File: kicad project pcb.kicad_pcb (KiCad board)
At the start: 2 copper layers, 35.3 x 38.9 mm, 11 parts, among them J1 Jack-DC, J2 Screw_Terminal_01x02, Q1 2N7000

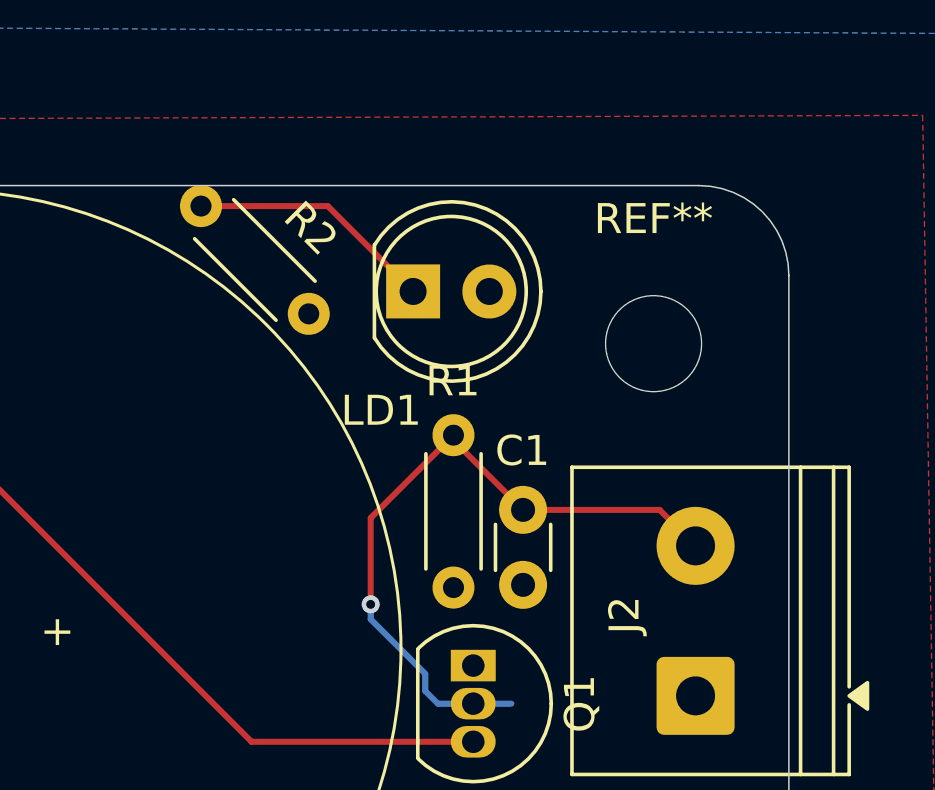
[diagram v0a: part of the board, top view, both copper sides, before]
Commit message: Update LED and screenshots
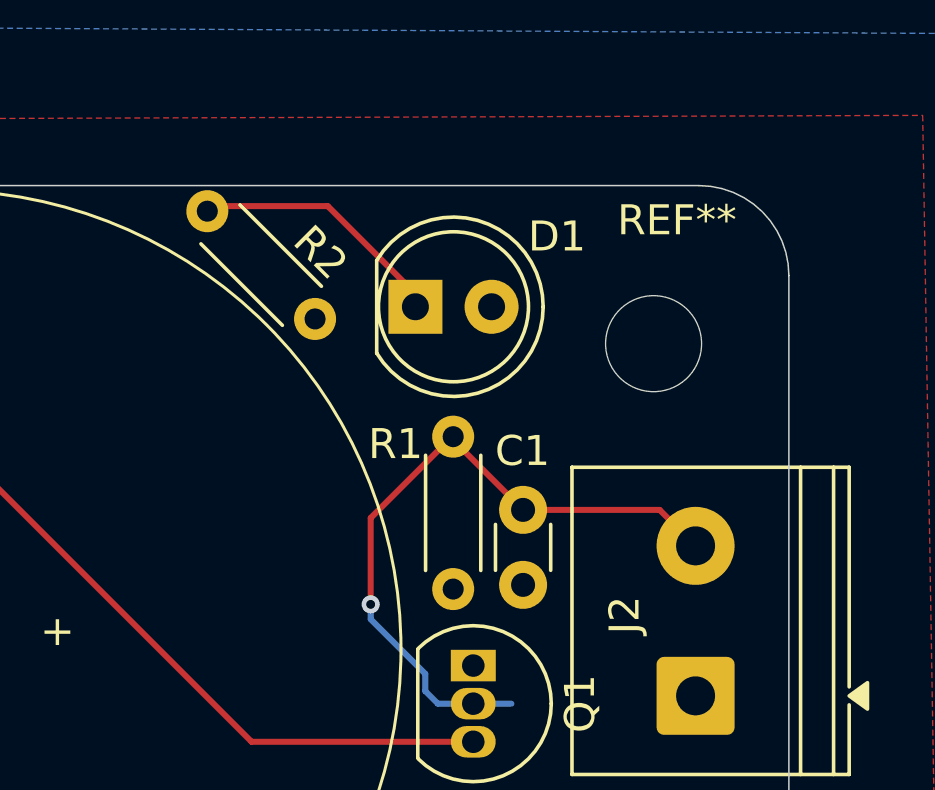
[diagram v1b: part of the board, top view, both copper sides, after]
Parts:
- removed LD1: SPL_PL90, LED_THT:LED_D5.0mm
- added D1: LED, LED_THT:LED_D5.0mm, F.Cu at (147.8, 83.0)
- moved R2 0.27 mm to (140.8, 79.8)
- moved R1 0.05 mm to (149.0, 87.3)
